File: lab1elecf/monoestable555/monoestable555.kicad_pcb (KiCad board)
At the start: 2 copper layers, 50 x 50 mm, 10 parts, among them J1 Conn_01x02, J2 Conn_01x02, J3 Conn_01x02, U1 LM555xM

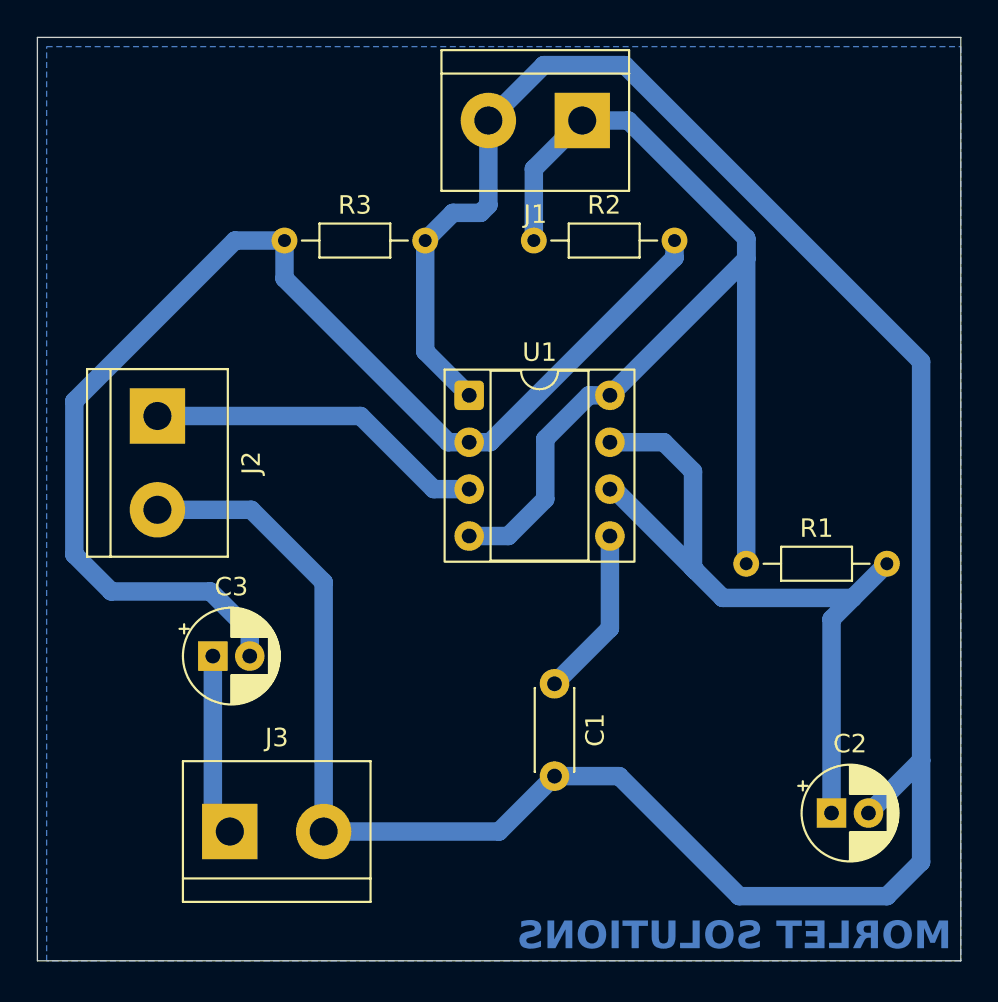
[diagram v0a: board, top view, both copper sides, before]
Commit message: VCC Y GND
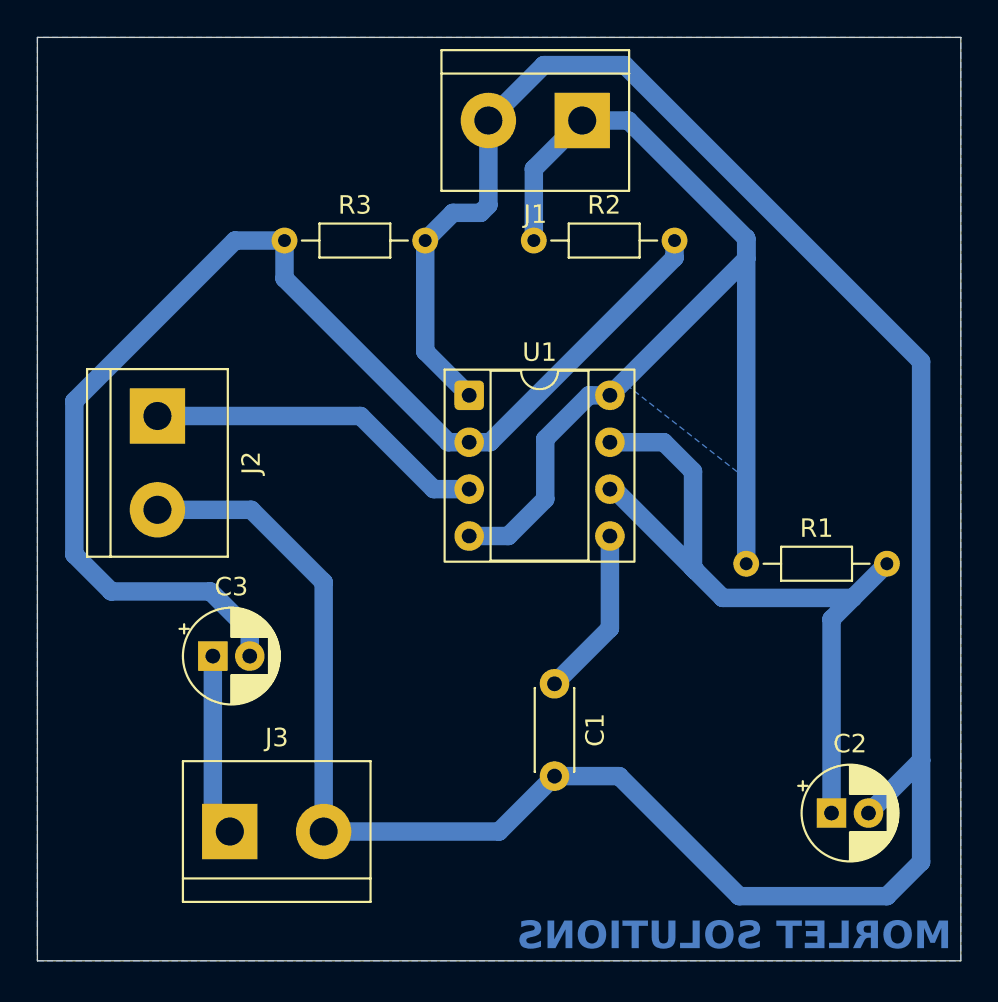
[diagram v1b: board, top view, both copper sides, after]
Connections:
- net Net-(J1-Pin_1) renamed VCC
- net Net-(J1-Pin_2) renamed GND
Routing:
- added copper zone on B.Cu, net GND
- added copper zone on B.Cu, net VCC
- removed copper zone on B.Cu, net (none)
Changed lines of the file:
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@@
 	(net 0 "")
 	(net 1 "Net-(U1-CV)")
-	(net 2 "Net-(J1-Pin_2)")
+	(net 2 "GND")
 	(net 3 "Net-(U1-DIS)")
 	(net 4 "Net-(U1-TR)")
 	(net 5 "Net-(J3-Pin_1)")
-	(net 6 "Net-(J1-Pin_1)")
+	(net 6 "VCC")
 	(net 7 "Net-(J2-Pin_1)")
 	(footprint "Capacitor_THT:C_Disc_D4.3mm_W1.9mm_P5.00mm"
@@
 			(layers "*.Cu" "*.Mask")
 			(remove_unused_layers no)
-			(net 2 "Net-(J1-Pin_2)")
+			(net 2 "GND")
 			(pintype "passive")
 		)
@@
 			(layers "*.Cu" "*.Mask")
 			(remove_unused_layers no)
-			(net 6 "Net-(J1-Pin_1)")
+			(net 6 "VCC")
 			(pinfunction "Pin_1")
 			(pintype "passive")
@@
 			(layers "*.Cu" "*.Mask")
 			(remove_unused_layers no)
-			(net 2 "Net-(J1-Pin_2)")
+			(net 2 "GND")
 			(pinfunction "Pin_2")
 			(pintype "passive")
@@
 			(layers "*.Cu" "*.Mask")
 			(remove_unused_layers no)
-			(net 6 "Net-(J1-Pin_1)")
+			(net 6 "VCC")
 			(pintype "passive")
 		)
@@
 			(layers "*.Cu" "*.Mask")
 			(remove_unused_layers no)
-			(net 2 "Net-(J1-Pin_2)")
+			(net 2 "GND")
 			(pinfunction "Pin_2")
 			(pintype "passive")
@@
 			(layers "*.Cu" "*.Mask")
 			(remove_unused_layers no)
-			(net 2 "Net-(J1-Pin_2)")
+			(net 2 "GND")
 			(pinfunction "Pin_2")
 			(pintype "passive")
@@
 			(remove_unused_layers no)
 			(roundrect_rratio 0.15625)
-			(net 2 "Net-(J1-Pin_2)")
+			(net 2 "GND")
 			(pinfunction "GND")
 			(pintype "power_in")
@@
 			(layers "*.Cu" "*.Mask")
 			(remove_unused_layers no)
-			(net 6 "Net-(J1-Pin_1)")
+			(net 6 "VCC")
 			(pinfunction "R")
 			(pintype "input")
@@
 			(layers "*.Cu" "*.Mask")
 			(remove_unused_layers no)
-			(net 6 "Net-(J1-Pin_1)")
+			(net 6 "VCC")
 			(pinfunction "VCC")
 			(pintype "power_in")
@@
 			(layers "*.Cu" "*.Mask")
 			(remove_unused_layers no)
-			(net 2 "Net-(J1-Pin_2)")
+			(net 2 "GND")
 			(pintype "passive")
 		)
@@
 			(layers "*.Cu" "*.Mask")
 			(remove_unused_layers no)
-			(net 6 "Net-(J1-Pin_1)")
+			(net 6 "VCC")
 			(pintype "passive")
 		)
@@
 			(layers "*.Cu" "*.Mask")
 			(remove_unused_layers no)
-			(net 2 "Net-(J1-Pin_2)")
+			(net 2 "GND")
 			(pintype "passive")
 		)
@@
 	)
 	(zone
-		(net 0)
-		(net_name "")
+		(net 2)
+		(net_name "GND")
+		(layer "B.Cu")
+		(hatch edge 0.5)
+		(connect_pads
+			(clearance 0.5)
+		)
+		(min_thickness 0.25)
+		(filled_areas_thickness no)
+		(fill yes
+			(thermal_gap 0.5)
+			(thermal_bridge_width 0.5)
+		)
+		(polygon
+			(pts
+				(xy 130 90) (xy 130 40) (xy 80 40) (xy 80 90)
+			)
+		)
+	)
+	(zone
+		(net 6)
+		(net_name "VCC")
 		(layer "B.Cu")
 		(hatch edge 0.5)
+		(priority 1)
 		(connect_pads
 			(clearance 0.5)
@@
 			(thermal_gap 0.5)
 			(thermal_bridge_width 0.5)
-			(island_removal_mode 1)
-			(island_area_min 10)
 		)
 		(polygon
 			(pts
-				(xy 130 40.5) (xy 130 90) (xy 80.5 90) (xy 80.5 40.5)
+				(xy 118 62.5) (xy 118.38 52) (xy 111.5 58.5) (xy 118.5 64) (xy 118 62)
 			)
 		)
